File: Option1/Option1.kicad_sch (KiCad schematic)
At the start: 0 parts

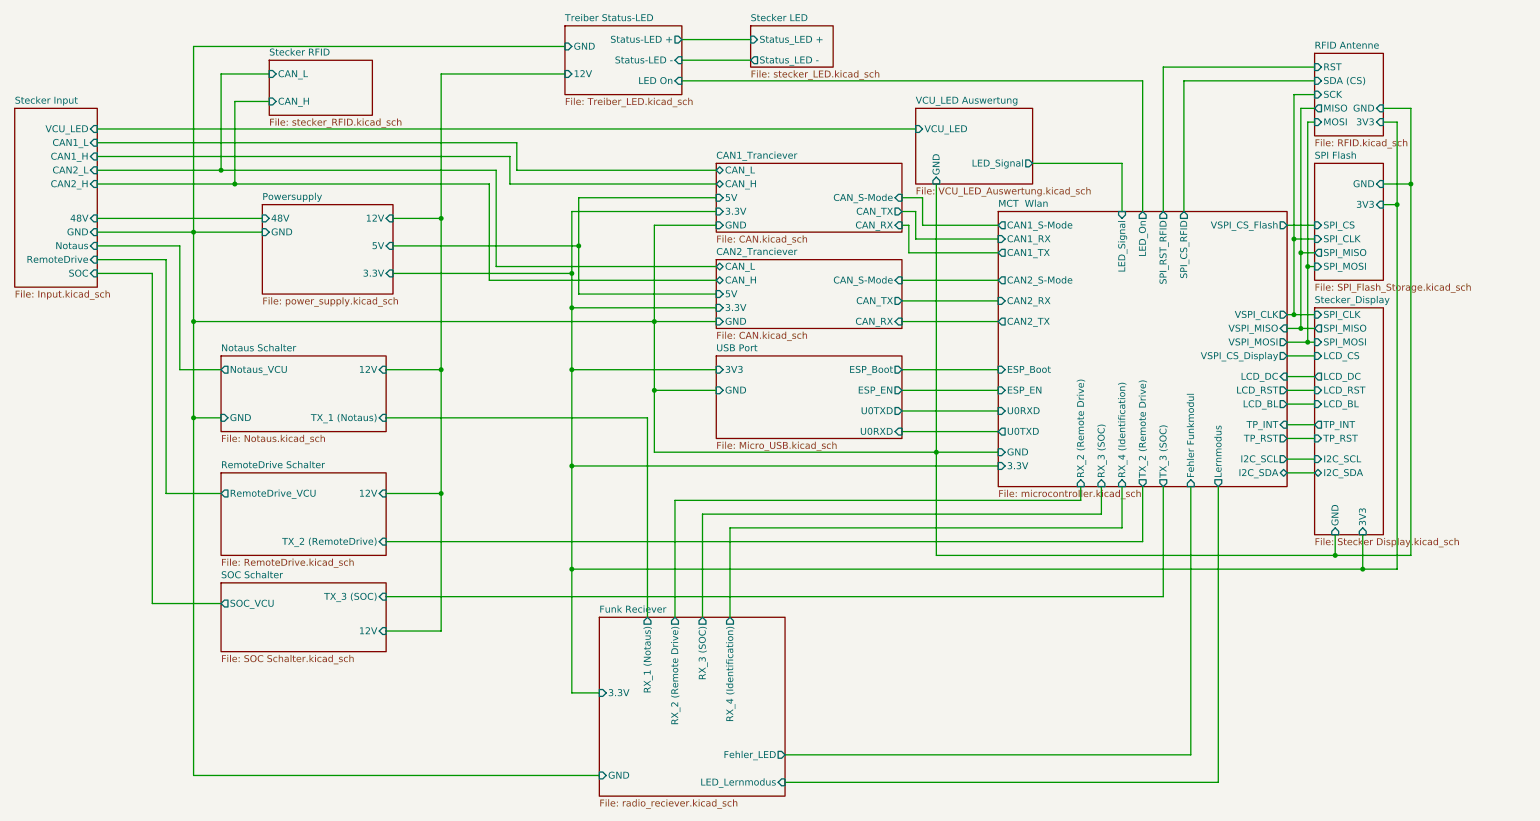
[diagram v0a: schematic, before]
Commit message: Erste issues eingearbeitet
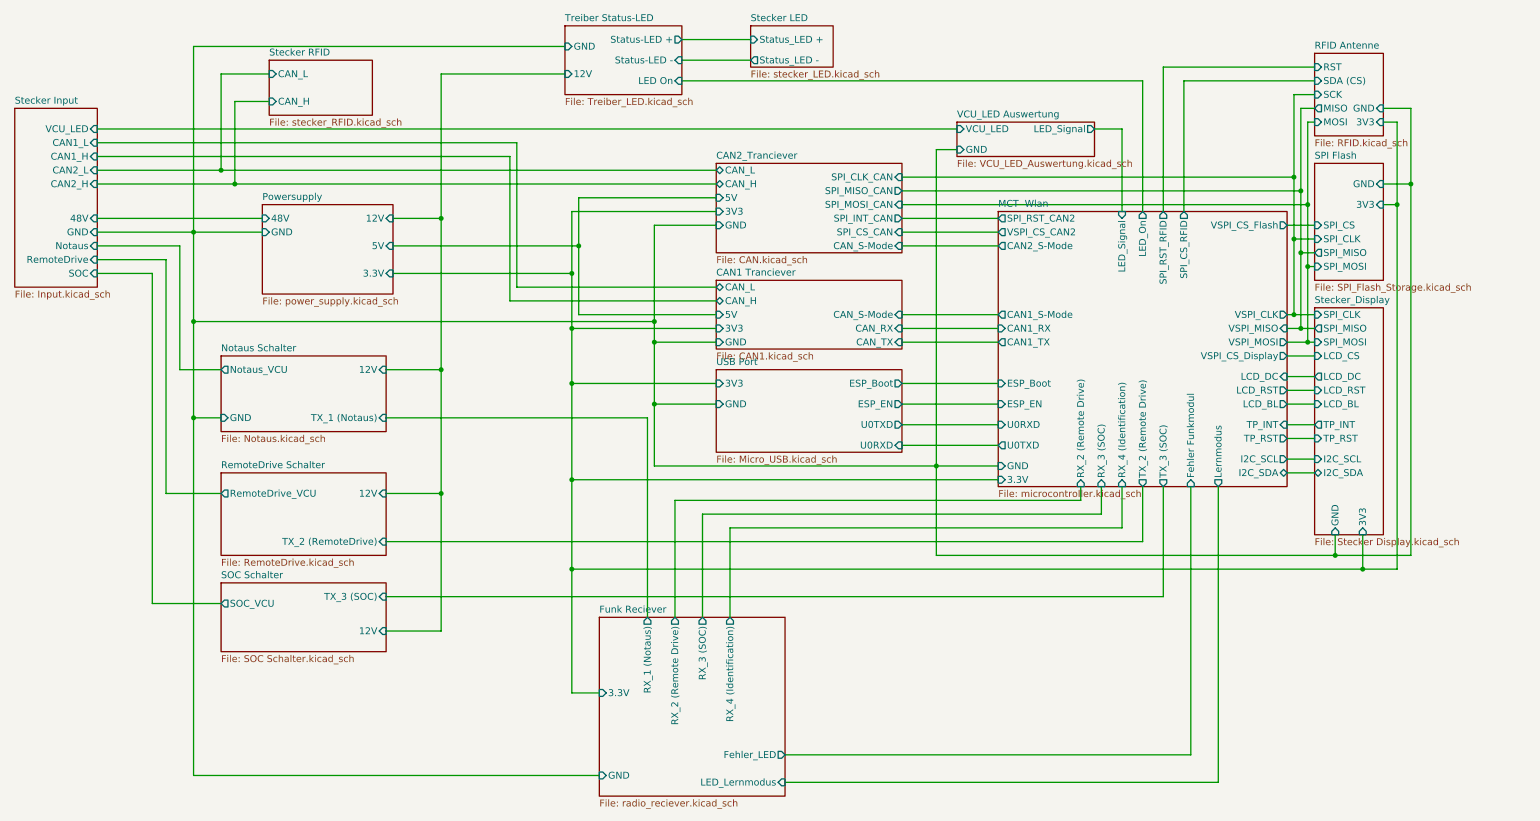
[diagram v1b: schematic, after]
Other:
- removed sheet CAN1_Tranciever
- added sheet CAN1 Tranciever (CAN1.kicad_sch)
- sheet CAN2_Tranciever ports: added 3V3, SPI_CLK_CAN, SPI_CS_CAN, SPI_INT_CAN, SPI_MISO_CAN, SPI_MOSI_CAN; removed 3.3V, CAN_RX, CAN_TX
- sheet MCT  Wlan ports: added SPI_RST_CAN2, VSPI_CS_CAN2; removed CAN2_RX, CAN2_TX
